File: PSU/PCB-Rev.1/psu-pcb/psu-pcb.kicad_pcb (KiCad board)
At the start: 2 copper layers, 100 x 100 mm, 60 parts, among them J1 Conn_02x07_Odd_Even, J2 OSTTC022162, J3 OSTTC022162, J4 OSTTC022162, J5 OSTTC022162, J6 OSTTC022162, J7 OSTTC022162, J8 Conn_02x05_Odd_Even, Q1 2N7002, Q2 2N7002, Q3 2N7002, Q4 FQP27P06, Q5 2N7002, U1 PIC12F1501-IP, U2 ADS1110

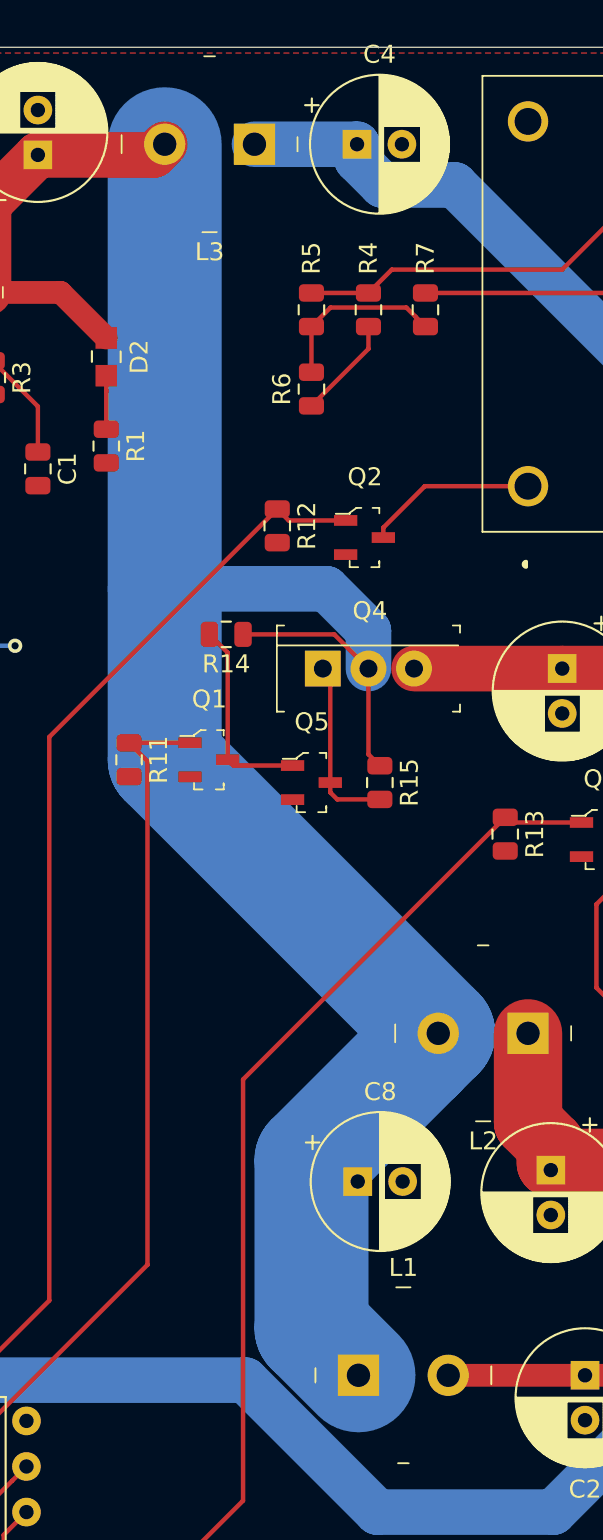
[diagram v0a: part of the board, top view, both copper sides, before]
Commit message: psu ready to be validated
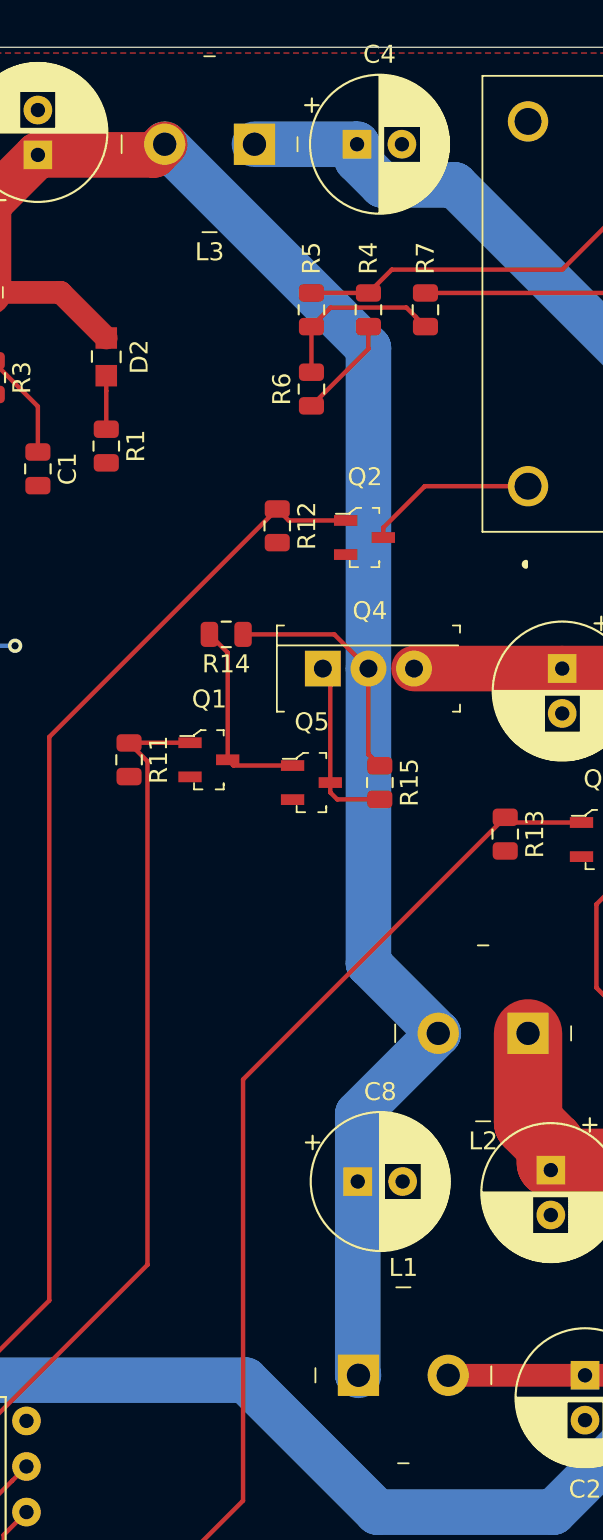
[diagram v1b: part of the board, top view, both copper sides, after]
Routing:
- net +12V: track 135.8 -> 119.2 mm
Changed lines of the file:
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@@
-(kicad_pcb (version 20171130) (host pcbnew 5.0.2+dfsg1-1~bpo9+1)
+(kicad_pcb (version 20171130) (host pcbnew "(5.1.5)-3")
   (general
     (thickness 1.6)
     (drawings 6)
-    (tracks 213)
+    (tracks 211)
     (zones 0)
     (modules 60)
@@
     (38 B.Mask user)
     (39 F.Mask user)
-    (40 Dwgs.User user)
-    (41 Cmts.User user)
-    (42 Eco1.User user)
-    (43 Eco2.User user)
+    (40 Dwgs.User user hide)
+    (41 Cmts.User user hide)
+    (42 Eco1.User user hide)
+    (43 Eco2.User user hide)
     (44 Edge.Cuts user)
     (45 Margin user)
     (46 B.CrtYd user)
     (47 F.CrtYd user)
-    (48 B.Fab user)
-    (49 F.Fab user)
+    (48 B.Fab user hide)
+    (49 F.Fab user hide)
   )
   (setup
-    (last_trace_width 0.25)
+    (last_trace_width 2.54)
     (user_trace_width 1.27)
     (user_trace_width 2.54)
@@
     (zone_45_only no)
     (trace_min 0.2)
-    (segment_width 0.2)
-    (edge_width 0.15)
     (via_size 0.8)
     (via_drill 0.4)
@@
     (uvia_min_size 0.2)
     (uvia_min_drill 0.1)
+    (edge_width 0.15)
+    (segment_width 0.2)
     (pcb_text_width 0.3)
     (pcb_text_size 1.5 1.5)
@@
     (solder_mask_min_width 0.25)
     (aux_axis_origin 0 0)
-    (visible_elements FFFFFF7F)
+    (visible_elements 7FFFFFFF)
     (pcbplotparams
       (layerselection 0x010fc_ffffffff)
@@
   (gr_line (start 120 120) (end 120 20) (layer Edge.Cuts) (width 0.01))
   (gr_line (start 20 20) (end 20 120) (layer Edge.Cuts) (width 0.01))
-  (via (at 116.84 22.86) (size 3.81) (drill 2.54) (layers F.Cu B.Cu) (net 2))
-  (via (at 36.83 83.185) (size 0.8) (drill 0.4) (layers F.Cu B.Cu) (net 2))
-  (via (at 42.545 53.34) (size 0.8) (drill 0.4) (layers F.Cu B.Cu) (net 2))
   (segment (start 38.735 33.655) (end 34.925 29.845) (width 2.54) (layer F.Cu) (net 1))
   (segment (start 41.275 33.655) (end 38.735 33.655) (width 2.54) (layer F.Cu) (net 1))
   (segment (start 28.575 36.195) (end 34.925 29.845) (width 2.54) (layer B.Cu) (net 1))
   (segment (start 26.035 36.195) (end 28.575 36.195) (width 2.54) (layer B.Cu) (net 1))
+  (via (at 116.84 22.86) (size 3.81) (drill 2.54) (layers F.Cu B.Cu) (net 2))
+  (via (at 36.83 83.185) (size 0.8) (drill 0.4) (layers F.Cu B.Cu) (net 2))
+  (via (at 42.545 53.34) (size 0.8) (drill 0.4) (layers F.Cu B.Cu) (net 2))
   (segment (start 66.04 36.8) (end 66.04 35.56) (width 0.25) (layer F.Cu) (net 2))
   (segment (start 62.865 39.975) (end 66.04 36.8) (width 0.25) (layer F.Cu) (net 2))
@@
   (segment (start 63.915 55.025) (end 63.5 54.61) (width 0.25) (layer F.Cu) (net 8))
   (segment (start 63.915 60.96) (end 63.915 55.025) (width 0.25) (layer F.Cu) (net 8))
-  (segment (start 68.780001 76.079999) (end 69.93 74.93) (width 6.35) (layer B.Cu) (net 9))
-  (segment (start 62.865 81.995) (end 68.780001 76.079999) (width 6.35) (layer B.Cu) (net 9))
-  (segment (start 62.865 91.36) (end 62.865 81.995) (width 6.35) (layer B.Cu) (net 9))
-  (segment (start 65.485 93.98) (end 62.865 91.36) (width 6.35) (layer B.Cu) (net 9))
-  (segment (start 69.93 74.93) (end 54.69 59.69) (width 6.35) (layer B.Cu) (net 9))
   (segment (start 44.875 28.745) (end 47.625 25.995) (width 2.54) (layer F.Cu) (net 9))
   (segment (start 44.875 33.655) (end 44.875 28.745) (width 2.54) (layer F.Cu) (net 9))
@@
   (segment (start 64.135 52.705) (end 66.04 54.61) (width 0.25) (layer F.Cu) (net 9))
   (segment (start 59.055 52.705) (end 64.135 52.705) (width 0.25) (layer F.Cu) (net 9))
-  (segment (start 63.701002 50.165) (end 54.69 50.165) (width 2.54) (layer B.Cu) (net 9))
-  (segment (start 66.04 52.503998) (end 63.701002 50.165) (width 2.54) (layer B.Cu) (net 9))
-  (segment (start 66.04 54.61) (end 66.04 52.503998) (width 2.54) (layer B.Cu) (net 9))
-  (segment (start 54.69 59.69) (end 54.69 50.165) (width 6.35) (layer B.Cu) (net 9))
-  (segment (start 54.69 50.165) (end 54.69 25.4) (width 6.35) (layer B.Cu) (net 9))
+  (segment (start 66.04 36.75) (end 66.04 54.61) (width 2.54) (layer B.Cu) (net 9))
+  (segment (start 54.69 25.4) (end 66.04 36.75) (width 2.54) (layer B.Cu) (net 9))
+  (segment (start 66.04 71.04) (end 69.93 74.93) (width 2.54) (layer B.Cu) (net 9))
+  (segment (start 66.04 54.61) (end 66.04 71.04) (width 2.54) (layer B.Cu) (net 9))
+  (segment (start 65.445 79.415) (end 65.445 83.185) (width 2.54) (layer B.Cu) (net 9))
+  (segment (start 69.93 74.93) (end 65.445 79.415) (width 2.54) (layer B.Cu) (net 9))
+  (segment (start 65.445 93.94) (end 65.485 93.98) (width 2.54) (layer B.Cu) (net 9))
+  (segment (start 65.445 83.185) (end 65.445 93.94) (width 2.54) (layer B.Cu) (net 9))
   (segment (start 83.265 54.61) (end 76.835 54.61) (width 2.54) (layer F.Cu) (net 10))
   (segment (start 83.9 55.245) (end 83.265 54.61) (width 2.54) (layer F.Cu) (net 10))
